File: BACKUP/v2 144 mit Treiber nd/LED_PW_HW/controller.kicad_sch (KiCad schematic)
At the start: 20 parts, among them SW1 SW_MEC_5E, U2 STM32L031K6Tx, Y1 Crystal

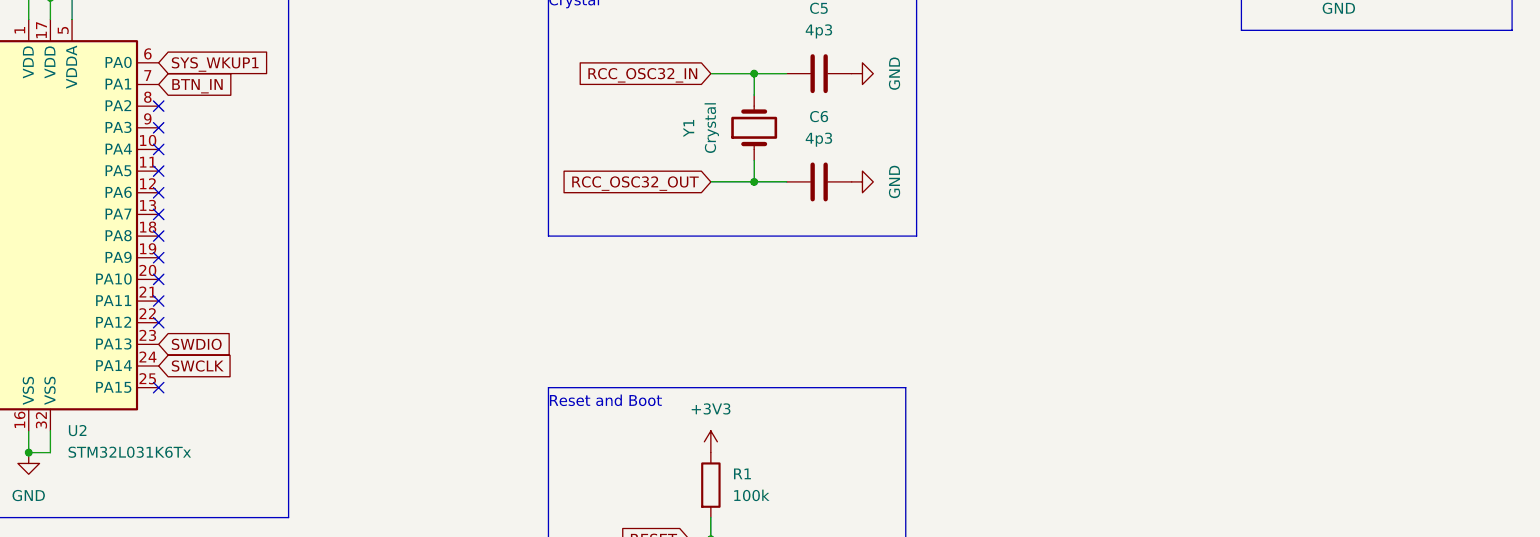
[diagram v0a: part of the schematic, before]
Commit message: new version
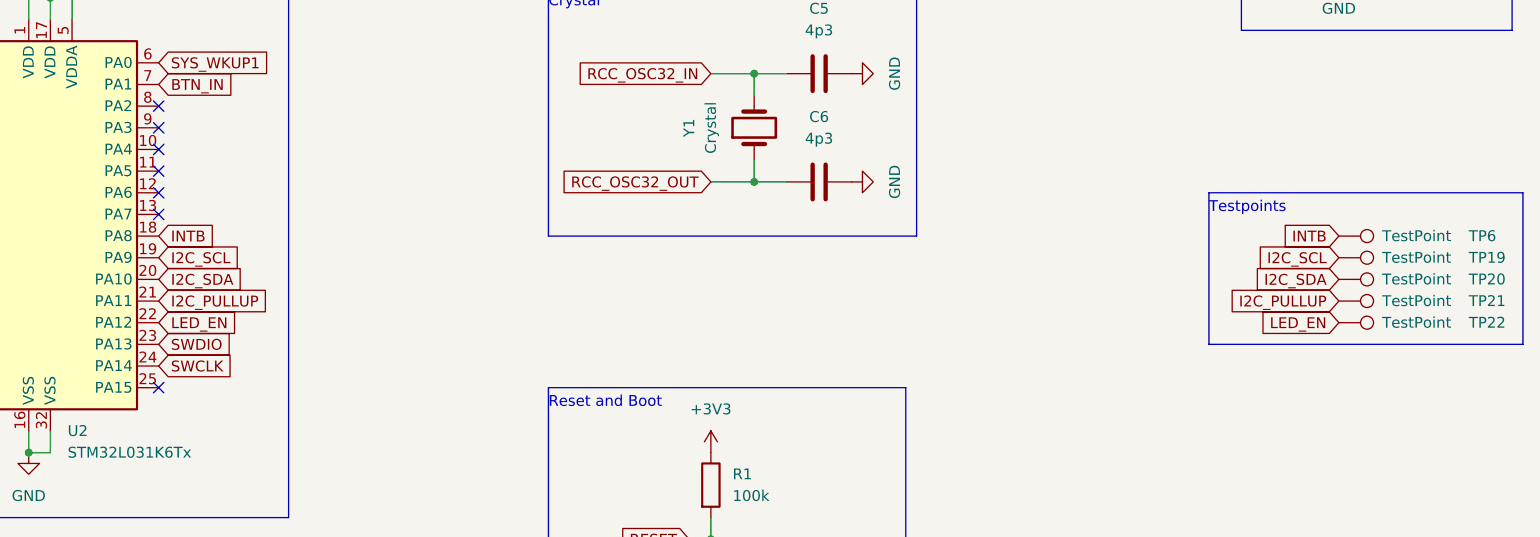
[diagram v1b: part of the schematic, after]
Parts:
- added TP19, TP20, TP21, TP22, TP6: TestPoint, TestPoint:TestPoint_Pad_D1.5mm, symbol Connector:TestPoint
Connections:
- net INTB: now reaches U2.18 (PA8)
- net INTB: now also TP6.1
- net I2C_SCL: now reaches U2.19 (PA9)
- net I2C_SCL: now also TP19.1
- net I2C_SDA: now reaches U2.20 (PA10)
- net I2C_SDA: now also TP20.1
- net I2C_PULLUP: now reaches U2.21 (PA11)
- net I2C_PULLUP: now also TP21.1
- net LED_EN: now reaches U2.22 (PA12)
- net LED_EN: now also TP22.1
- no-connect marks 19 -> 14
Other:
- note added: "Testpoints"
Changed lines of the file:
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@@
   (no_connect (at 73.66 113.03))
   (no_connect (at 73.66 80.01))
-  (no_connect (at 73.66 95.25))
-  (no_connect (at 73.66 97.79))
-  (no_connect (at 73.66 100.33))
-  (no_connect (at 73.66 102.87))
-  (no_connect (at 73.66 105.41))
   (no_connect (at 45.72 110.49))
   (no_connect (at 45.72 113.03))
@@
     (stroke (width 0) (type default) (color 0 0 0 0))
   )
+  (polyline (pts (xy 196.85 90.17) (xy 196.85 107.95))
+    (stroke (width 0) (type default) (color 0 0 0 0))
+  )
   (wire (pts (xy 138.43 88.9) (xy 143.51 88.9))
     (stroke (width 0) (type default) (color 0 0 0 0))
@@
     (stroke (width 0) (type default) (color 0 0 0 0))
   )
+  (polyline (pts (xy 233.68 107.95) (xy 233.68 90.17))
+    (stroke (width 0) (type default) (color 0 0 0 0))
+  )
   (wire (pts (xy 162.56 29.21) (xy 167.64 29.21))
     (stroke (width 0) (type default) (color 0 0 0 0))
@@
   )
   (wire (pts (xy 167.64 29.21) (xy 167.64 26.67))
+    (stroke (width 0) (type default) (color 0 0 0 0))
+  )
+  (polyline (pts (xy 196.85 90.17) (xy 233.68 90.17))
+    (stroke (width 0) (type default) (color 0 0 0 0))
+  )
+  (polyline (pts (xy 196.85 107.95) (xy 233.68 107.95))
     (stroke (width 0) (type default) (color 0 0 0 0))
   )
@@
     (effects (font (size 1.27 1.27)) (justify left bottom))
   )
+  (text "Testpoints" (at 196.85 92.71 0)
+    (effects (font (size 1.27 1.27)) (justify left bottom))
+  )
   (global_label "SYS_WKUP1" (shape input) (at 139.7 34.29 180) (fields_autoplaced)
     (effects (font (size 1.27 1.27)) (justify right))
@@
     )
   )
+  (global_label "LED_EN" (shape input) (at 212.09 105.41 180) (fields_autoplaced)
+    (effects (font (size 1.27 1.27)) (justify right))
+    (property "Intersheet References" "${INTERSHEET_REFS}" (id 0) (at 202.7826 105.3306 0)
+      (effects (font (size 1.27 1.27)) (justify right) hide)
+    )
+  )
   (global_label "RCC_OSC32_OUT" (shape input) (at 45.72 92.71 180) (fields_autoplaced)
     (effects (font (size 1.27 1.27)) (justify right))
@@
     (property "Intersheet References" "${INTERSHEET_REFS}" (id 0) (at 203.4479 60.8806 0)
       (effects (font (size 1.27 1.27)) (justify right) hide)
+    )
+  )
+  (global_label "INTB" (shape input) (at 73.66 95.25 0) (fields_autoplaced)
+    (effects (font (size 1.27 1.27)) (justify left))
+    (property "Intersheet References" "${INTERSHEET_REFS}" (id 0) (at 80.246 95.1706 0)
+      (effects (font (size 1.27 1.27)) (justify left) hide)
+    )
+  )
+  (global_label "LED_EN" (shape input) (at 73.66 105.41 0) (fields_autoplaced)
+    (effects (font (size 1.27 1.27)) (justify left))
+    (property "Intersheet References" "${INTERSHEET_REFS}" (id 0) (at 82.9674 105.3306 0)
+      (effects (font (size 1.27 1.27)) (justify left) hide)
+    )
+  )
+  (global_label "I2C_SCL" (shape input) (at 73.66 97.79 0) (fields_autoplaced)
+    (effects (font (size 1.27 1.27)) (justify left))
+    (property "Intersheet References" "${INTERSHEET_REFS}" (id 0) (at 83.6326 97.7106 0)
+      (effects (font (size 1.27 1.27)) (justify left) hide)
     )
   )
@@
     )
   )
+  (global_label "I2C_SCL" (shape input) (at 212.09 97.79 180) (fields_autoplaced)
+    (effects (font (size 1.27 1.27)) (justify right))
+    (property "Intersheet References" "${INTERSHEET_REFS}" (id 0) (at 202.1174 97.7106 0)
+      (effects (font (size 1.27 1.27)) (justify right) hide)
+    )
+  )
+  (global_label "I2C_SDA" (shape input) (at 73.66 100.33 0) (fields_autoplaced)
+    (effects (font (size 1.27 1.27)) (justify left))
+    (property "Intersheet References" "${INTERSHEET_REFS}" (id 0) (at 83.6931 100.2506 0)
+      (effects (font (size 1.27 1.27)) (justify left) hide)
+    )
+  )
+  (global_label "I2C_SDA" (shape input) (at 212.09 100.33 180) (fields_autoplaced)
+    (effects (font (size 1.27 1.27)) (justify right))
+    (property "Intersheet References" "${INTERSHEET_REFS}" (id 0) (at 202.0569 100.2506 0)
+      (effects (font (size 1.27 1.27)) (justify right) hide)
+    )
+  )
   (global_label "BOOT" (shape input) (at 135.89 133.35 180) (fields_autoplaced)
     (effects (font (size 1.27 1.27)) (justify right))
@@
     )
   )
+  (global_label "INTB" (shape input) (at 212.09 95.25 180) (fields_autoplaced)
+    (effects (font (size 1.27 1.27)) (justify right))
+    (property "Intersheet References" "${INTERSHEET_REFS}" (id 0) (at 205.504 95.3294 0)
+      (effects (font (size 1.27 1.27)) (justify right) hide)
+    )
+  )
   (global_label "SWDIO" (shape input) (at 212.09 58.42 180) (fields_autoplaced)
     (effects (font (size 1.27 1.27)) (justify right))
@@
     )
   )
+  (global_label "I2C_PULLUP" (shape input) (at 73.66 102.87 0) (fields_autoplaced)
+    (effects (font (size 1.27 1.27)) (justify left))
+    (property "Intersheet References" "${INTERSHEET_REFS}" (id 0) (at 87.3821 102.7906 0)
+      (effects (font (size 1.27 1.27)) (justify left) hide)
+    )
+  )
   (global_label "BTN_IN" (shape input) (at 139.7 41.91 180) (fields_autoplaced)
     (effects (font (size 1.27 1.27)) (justify right))
@@
     )
   )
+  (global_label "I2C_PULLUP" (shape input) (at 212.09 102.87 180) (fields_autoplaced)
+    (effects (font (size 1.27 1.27)) (justify right))
+    (property "Intersheet References" "${INTERSHEET_REFS}" (id 0) (at 198.3679 102.7906 0)
+      (effects (font (size 1.27 1.27)) (justify right) hide)
+    )
+  )
   (global_label "BTN_IN" (shape input) (at 139.7 26.67 180) (fields_autoplaced)
     (effects (font (size 1.27 1.27)) (justify right))
@@
     (pin "1")
   )
+  (symbol (lib_id "Connector:TestPoint") (at 212.09 95.25 270) (unit 1)
+    (in_bom yes) (on_board yes)
+    (property "Reference" "TP6" (id 0) (at 227.33 95.25 90)
+      (effects (font (size 1.27 1.27)) (justify left))
+    )
+    (property "Value" "TestPoint" (id 1) (at 217.17 95.25 90)
+      (effects (font (size 1.27 1.27)) (justify left))
+    )
+    (property "Footprint" "TestPoint:TestPoint_Pad_D1.5mm" (id 2) (at 212.09 100.33 0)
+      (effects (font (size 1.27 1.27)) hide)
+    )
+    (property "Datasheet" "~" (id 3) (at 212.09 100.33 0)
+      (effects (font (size 1.27 1.27)) hide)
+    )
+    (pin "1")
+  )
   (symbol (lib_id "power:+3V3") (at 53.34 40.64 0) (unit 1)
     (in_bom yes) (on_board yes) (fields_autoplaced)
@@
     (pin "2")
   )
+  (symbol (lib_id "Connector:TestPoint") (at 212.09 97.79 270) (unit 1)
+    (in_bom yes) (on_board yes)
+    (property "Reference" "TP19" (id 0) (at 227.33 97.79 90)
+      (effects (font (size 1.27 1.27)) (justify left))
+    )
+    (property "Value" "TestPoint" (id 1) (at 217.17 97.79 90)
+      (effects (font (size 1.27 1.27)) (justify left))
+    )
+    (property "Footprint" "TestPoint:TestPoint_Pad_D1.5mm" (id 2) (at 212.09 102.87 0)
+      (effects (font (size 1.27 1.27)) hide)
+    )
+    (property "Datasheet" "~" (id 3) (at 212.09 102.87 0)
+      (effects (font (size 1.27 1.27)) hide)
+    )
+    (pin "1")
+  )
   (symbol (lib_id "Device:C") (at 27.94 44.45 0) (unit 1)
     (in_bom yes) (on_board yes) (fields_autoplaced)
@@
     (pin "1")
     (pin "2")
+  )
+  (symbol (lib_id "Connector:TestPoint") (at 212.09 105.41 270) (unit 1)
+    (in_bom yes) (on_board yes)
+    (property "Reference" "TP22" (id 0) (at 227.33 105.41 90)
+      (effects (font (size 1.27 1.27)) (justify left))
+    )
+    (property "Value" "TestPoint" (id 1) (at 217.17 105.41 90)
+      (effects (font (size 1.27 1.27)) (justify left))
+    )
+    (property "Footprint" "TestPoint:TestPoint_Pad_D1.5mm" (id 2) (at 212.09 110.49 0)
+      (effects (font (size 1.27 1.27)) hide)
+    )
+    (property "Datasheet" "~" (id 3) (at 212.09 110.49 0)
+      (effects (font (size 1.27 1.27)) hide)
+    )
+    (pin "1")
+  )
+  (symbol (lib_id "Connector:TestPoint") (at 212.09 100.33 270) (unit 1)
+    (in_bom yes) (on_board yes)
+    (property "Reference" "TP20" (id 0) (at 227.33 100.33 90)
+      (effects (font (size 1.27 1.27)) (justify left))
+    )
+    (property "Value" "TestPoint" (id 1) (at 217.17 100.33 90)
+      (effects (font (size 1.27 1.27)) (justify left))
+    )
+    (property "Footprint" "TestPoint:TestPoint_Pad_D1.5mm" (id 2) (at 212.09 105.41 0)
+      (effects (font (size 1.27 1.27)) hide)
+    )
+    (property "Datasheet" "~" (id 3) (at 212.09 105.41 0)
+      (effects (font (size 1.27 1.27)) hide)
+    )
+    (pin "1")
   )
   (symbol (lib_id "Device:C") (at 53.34 44.45 0) (unit 1)
@@
     (pin "4")
   )
+  (symbol (lib_id "Connector:TestPoint") (at 212.09 102.87 270) (unit 1)
+    (in_bom yes) (on_board yes)
+    (property "Reference" "TP21" (id 0) (at 227.33 102.87 90)
+      (effects (font (size 1.27 1.27)) (justify left))
+    )
+    (property "Value" "TestPoint" (id 1) (at 217.17 102.87 90)
+      (effects (font (size 1.27 1.27)) (justify left))
+    )
+    (property "Footprint" "TestPoint:TestPoint_Pad_D1.5mm" (id 2) (at 212.09 107.95 0)
+      (effects (font (size 1.27 1.27)) hide)
+    )
+    (property "Datasheet" "~" (id 3) (at 212.09 107.95 0)
+      (effects (font (size 1.27 1.27)) hide)
+    )
+    (pin "1")
+  )
   (symbol (lib_id "power:GND") (at 142.24 52.07 0) (unit 1)
